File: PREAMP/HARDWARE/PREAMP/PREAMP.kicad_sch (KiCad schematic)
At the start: 1 part, among them U1 TL074

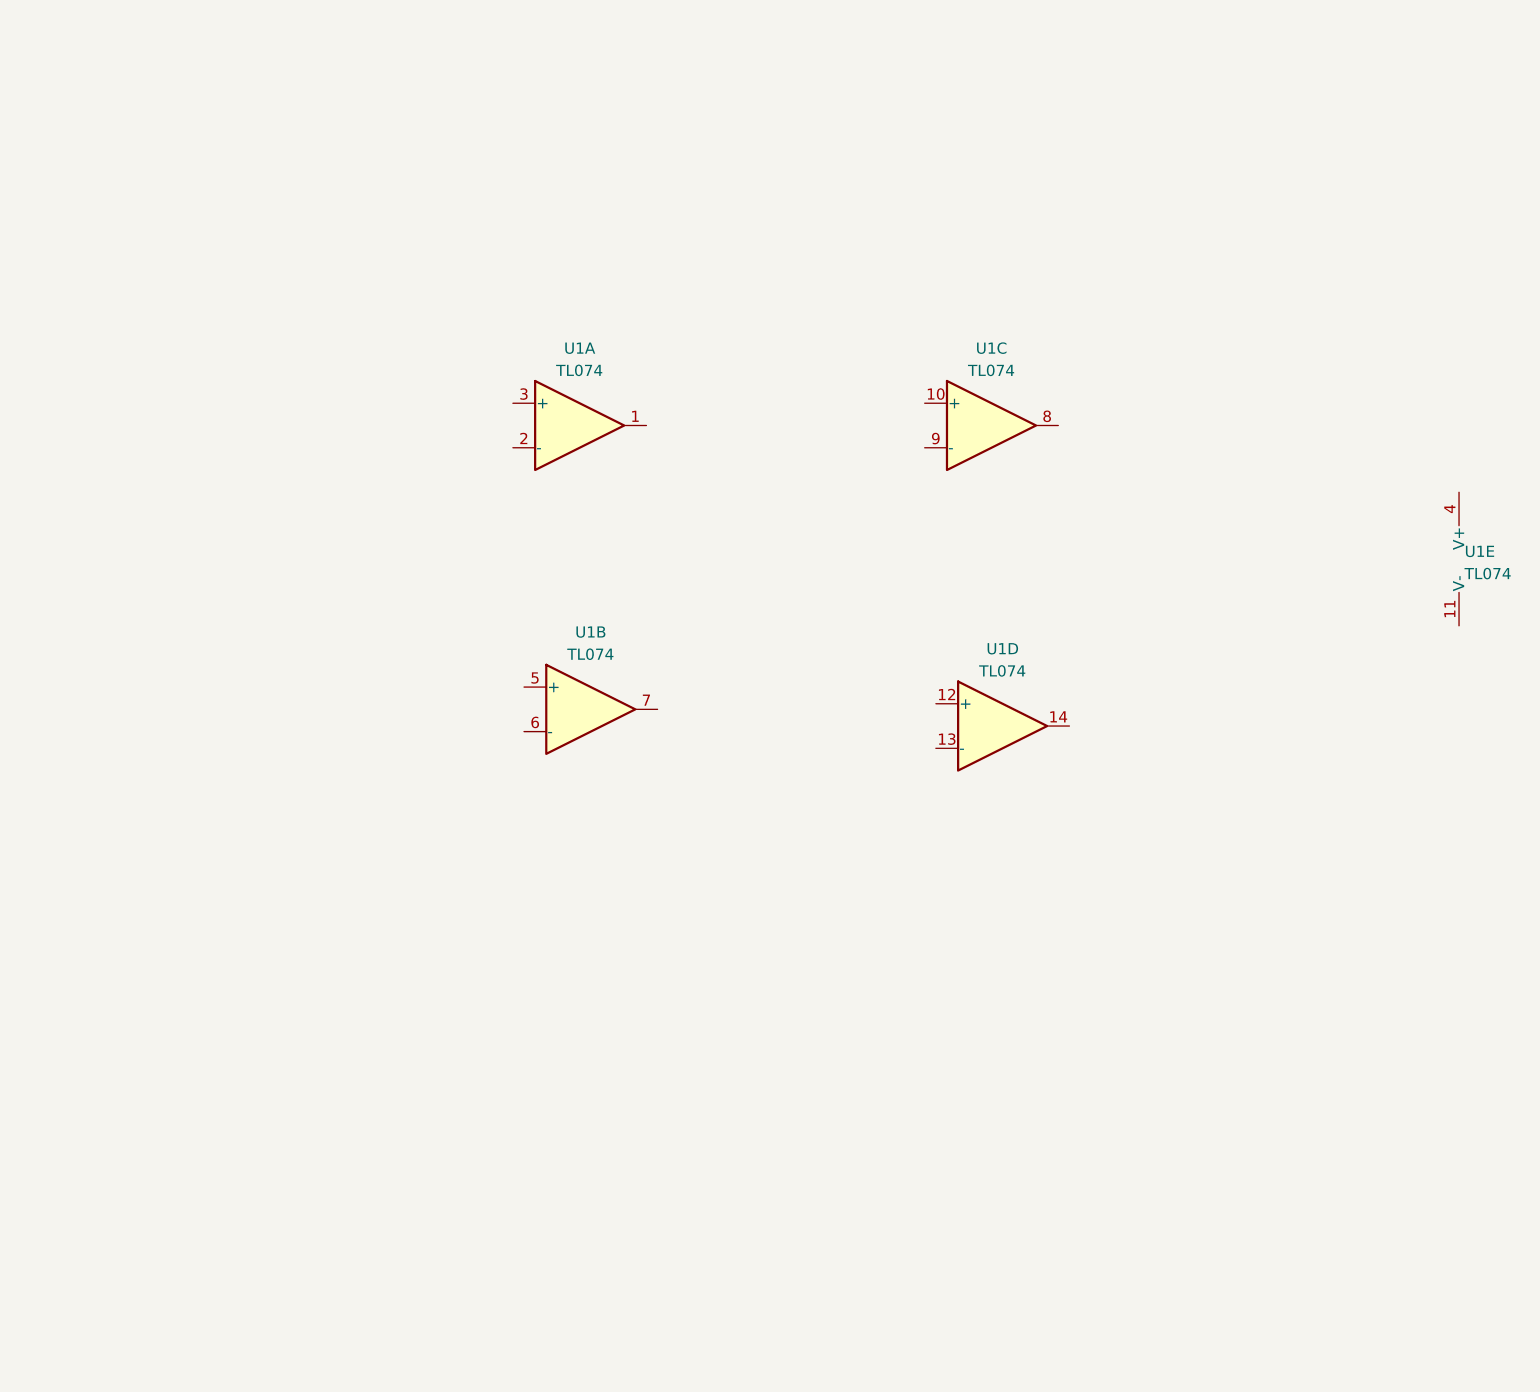
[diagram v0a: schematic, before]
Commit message: Schematic V01
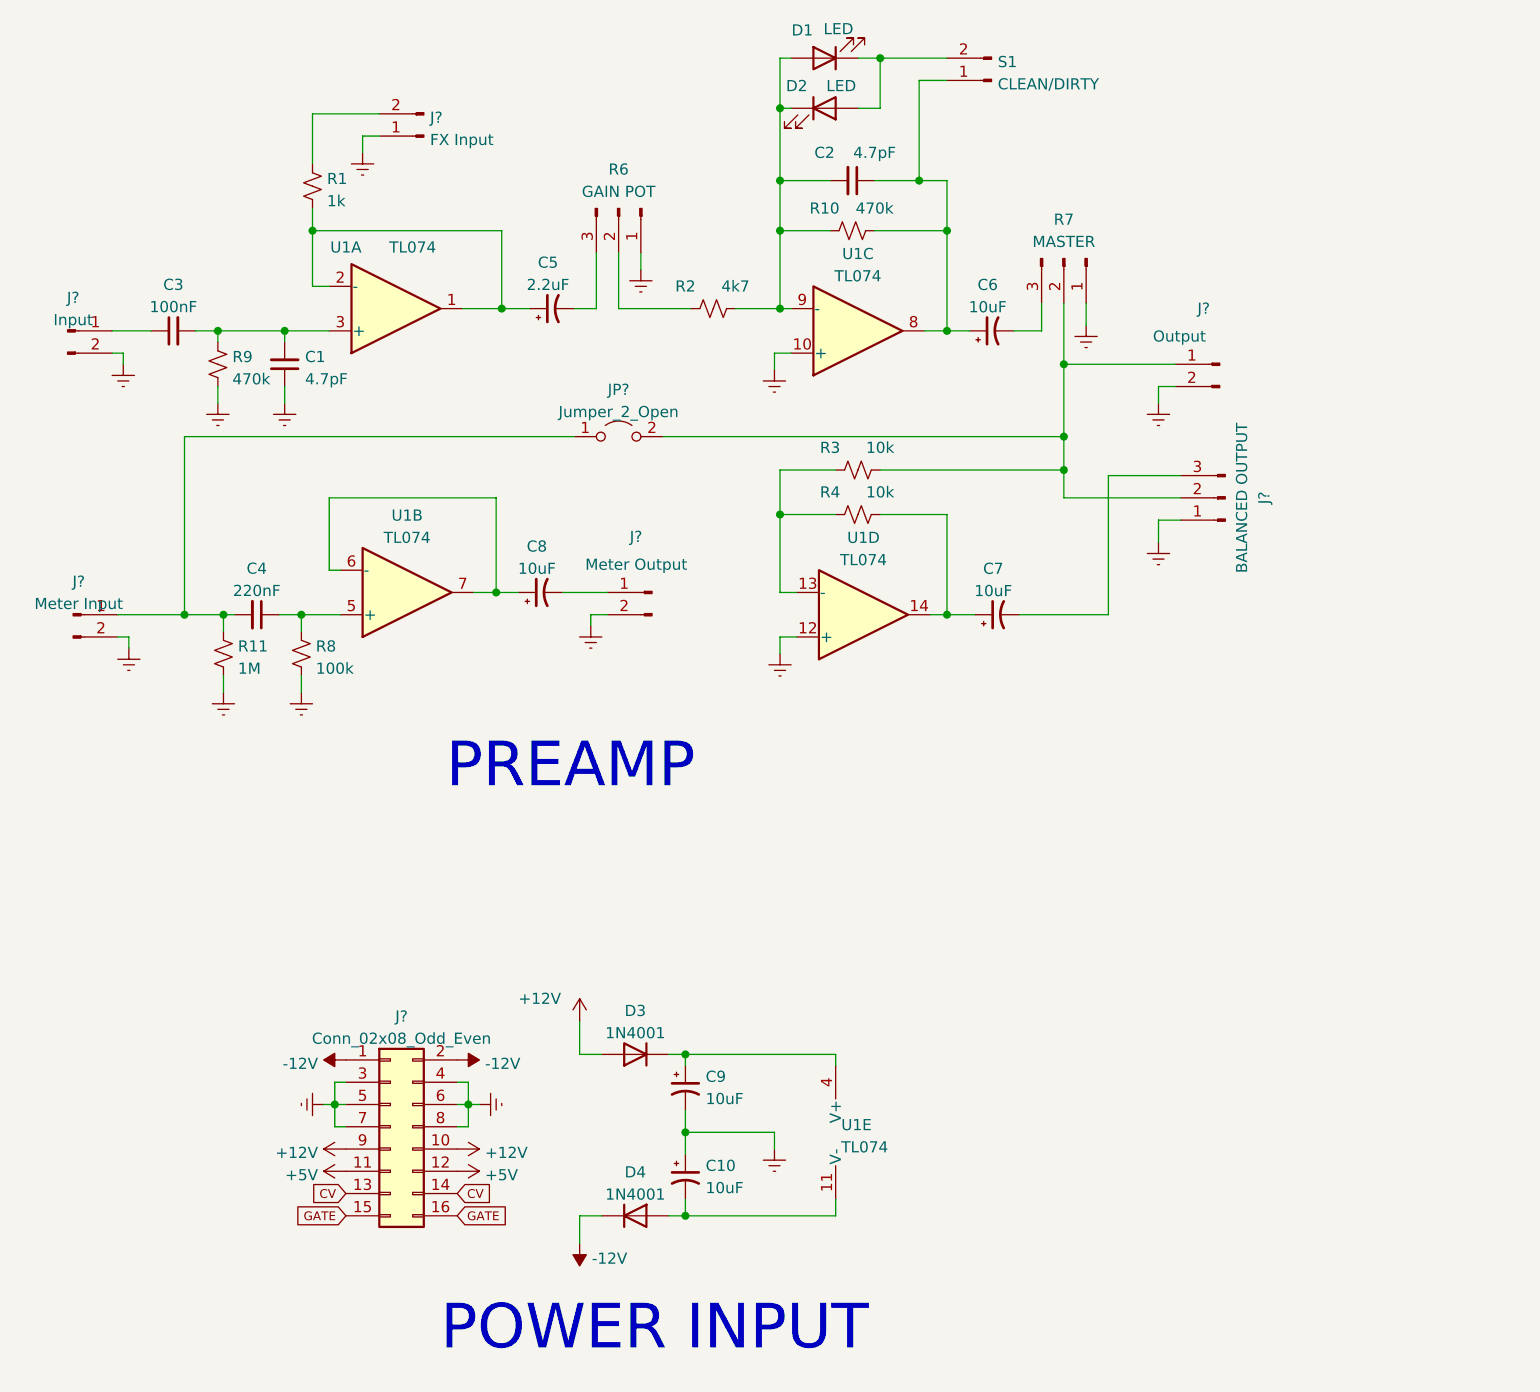
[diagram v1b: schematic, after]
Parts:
- added C1, C2: 4.7pF, Capacitor_THT:C_Disc_D5.0mm_W2.5mm_P5.00mm, symbol Device:C_Small
- added C10, C6, C7, C8, C9: 10uF, Capacitor_THT:CP_Radial_D8.0mm_P3.80mm, symbol Device:C_Polarized_Small_US
- added C3: 100nF, Capacitor_THT:C_Disc_D5.0mm_W2.5mm_P5.00mm, symbol Device:C_Small
- added C4: 220nF, Capacitor_THT:C_Disc_D5.0mm_W2.5mm_P5.00mm, symbol Device:C_Small
- added C5: 2.2uF, Capacitor_THT:CP_Radial_D8.0mm_P3.80mm, symbol Device:C_Polarized_Small_US
- added D1, D2: LED, symbol Device:LED
- added D3, D4: 1N4001, Diode_THT:D_DO-41_SOD81_P10.16mm_Horizontal, symbol Diode:1N4001
- added J?: FX Input, Connector_Molex:Molex_SL_171971-0002_1x02_P2.54mm_Vertical, symbol Connector:Conn_01x02_Male
- added J?: Input, Connector_Molex:Molex_SL_171971-0002_1x02_P2.54mm_Vertical, symbol Connector:Conn_01x02_Male
- added J?: Meter Output, Connector_Molex:Molex_SL_171971-0002_1x02_P2.54mm_Vertical, symbol Connector:Conn_01x02_Male
- added J?: Output, Connector_Molex:Molex_SL_171971-0002_1x02_P2.54mm_Vertical, symbol Connector:Conn_01x02_Male
- added J?: BALANCED OUTPUT, symbol Connector:Conn_01x03_Male
- added J?: Meter Input, Connector_Molex:Molex_SL_171971-0002_1x02_P2.54mm_Vertical, symbol Connector:Conn_01x02_Male
- added J?: Conn_02x08_Odd_Even, Connector_IDC:IDC-Header_2x08_P2.54mm_Vertical, symbol Connector_Generic:Conn_02x08_Odd_Even
- added JP?: Jumper_2_Open, Connector_PinSocket_2.54mm:PinSocket_1x02_P2.54mm_Vertical, symbol Jumper:Jumper_2_Open
- added R1: 1k, Resistor_THT:R_Axial_DIN0207_L6.3mm_D2.5mm_P7.62mm_Horizontal, symbol Device:R_Small_US
- added R10, R9: 470k, Resistor_THT:R_Axial_DIN0207_L6.3mm_D2.5mm_P7.62mm_Horizontal, symbol Device:R_Small_US
- added R11: 1M, Resistor_THT:R_Axial_DIN0207_L6.3mm_D2.5mm_P7.62mm_Horizontal, symbol Device:R_Small_US
- added R2: 4k7, Resistor_THT:R_Axial_DIN0207_L6.3mm_D2.5mm_P7.62mm_Horizontal, symbol Device:R_Small_US
- added R3, R4: 10k, Resistor_THT:R_Axial_DIN0207_L6.3mm_D2.5mm_P7.62mm_Horizontal, symbol Device:R_Small_US
- added R6: GAIN POT, symbol Connector:Conn_01x03_Male
- added R7: MASTER, symbol Connector:Conn_01x03_Male
- added R8: 100k, Resistor_THT:R_Axial_DIN0207_L6.3mm_D2.5mm_P7.62mm_Horizontal, symbol Device:R_Small_US
- added S1: CLEAN/DIRTY, Connector_Molex:Molex_SL_171971-0002_1x02_P2.54mm_Vertical, symbol Connector:Conn_01x02_Male
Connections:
- net at U1.5 (+): now also C4.1, R8.1
- net at U1.6 (-): now also U1.7, C8.1
- net Earth: now reaches U1.10 (+)
- net Earth: now also U1.12 (+), C1.1, C10.1, C9.2, J?.1 (Pin_1), J?.1 (Pin_1), J?.2 (Pin_2), J?.2 (Pin_2), J?.2 (Pin_2), J?.2 (Pin_2), J?.3 (Pin_3), J?.4 (Pin_4), J?.5 (Pin_5), J?.6 (Pin_6), J?.7 (Pin_7), J?.8 (Pin_8), R11.2, R6.1 (Pin_1), R7.1 (Pin_1), R8.2, R9.2
- net at U1.8: now also C2.1, C6.1, R10.2, S1.1 (Pin_1)
- net at U1.9 (-): now also C2.2, D1.2 (A), D2.1 (K), R10.1, R2.2
- net at U1.13 (-): now also R3.1, R4.1
- net at U1.14: now also C7.1, R4.2
- net at U1.11 (V-): now also C10.2, D4.2 (A)
- net at U1.4 (V+): now also C9.1, D3.1 (K)
- net at U1.1: now also U1.2 (-), C5.1, R1.2
- net at U1.3 (+): now also C1.2, C3.2, R9.1
- new net: C3.1, J?.1 (Pin_1)
- new net: C5.2, R6.3 (Pin_3)
- new net: J?.2 (Pin_2), R1.1
- new net: C6.2, R7.3 (Pin_3)
- new net: C4.2, J?.1 (Pin_1), JP?.1 (A), R11.1
- new net: J?.1 (Pin_1), J?.2 (Pin_2), JP?.2 (B), R3.2, R7.2 (Pin_2)
- new net: C8.2, J?.1 (Pin_1)
- new net: R2.1, R6.2 (Pin_2)
- new net: D1.1 (K), D2.2 (A), S1.2 (Pin_2)
- new net: C7.2, J?.3 (Pin_3)
- new net +12V: D3.2 (A), J?.10 (Pin_10), J?.9 (Pin_9)
- new net +5V: J?.11 (Pin_11), J?.12 (Pin_12)
- new net -12V: D4.1 (K), J?.1 (Pin_1), J?.2 (Pin_2)
- new net CV: J?.13 (Pin_13), J?.14 (Pin_14)
- new net GATE: J?.15 (Pin_15), J?.16 (Pin_16)
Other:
- note added: "POWER INPUT"
- note added: "PREAMP"
- moved on the sheet: U1A, U1B, U1C, U1D, U1E
